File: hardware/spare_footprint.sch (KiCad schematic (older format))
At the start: 32 parts

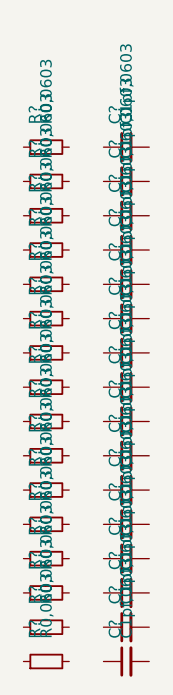
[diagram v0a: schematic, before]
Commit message: update,
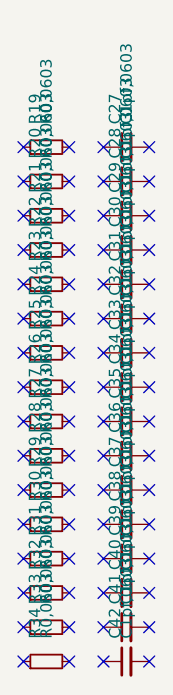
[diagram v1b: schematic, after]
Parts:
- gave numbers to parts that had none: 32
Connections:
- no-connect marks 0 -> 64

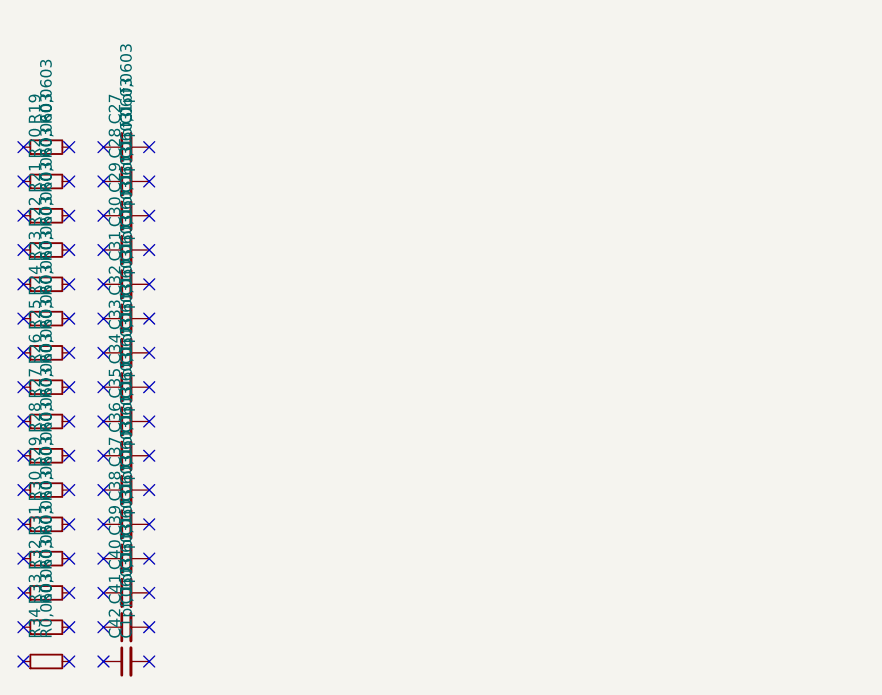
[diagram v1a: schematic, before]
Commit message: update,
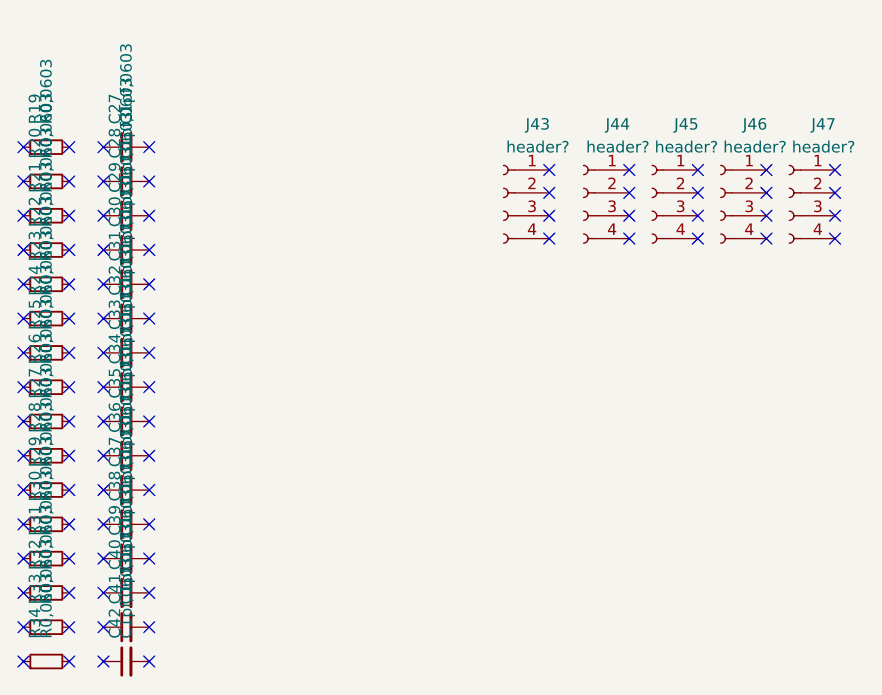
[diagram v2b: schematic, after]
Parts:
- added J43, J44, J45, J46, J47: header?, symbol Connector:Conn_01x04_Female
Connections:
- no-connect marks 64 -> 84
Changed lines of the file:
@@
 NoConn ~ 1650 3450
 NoConn ~ 1650 3600
+$Comp
+L Connector:Conn_01x04_Female J43
+U 1 1 5CFDD06D
+P 3550 1550
+F 0 "J43" H 3400 1850 50  0000 C CNN
+F 1 "header?" H 3400 1750 50  0000 C CNN
+F 2 "" H 3550 1550 50  0001 C CNN
+F 3 "~" H 3550 1550 50  0001 C CNN
+	1    3550 1550
+	-1   0    0    -1
+$EndComp
+NoConn ~ 3750 1450
+NoConn ~ 3750 1550
+NoConn ~ 3750 1650
+NoConn ~ 3750 1750
+$Comp
+L Connector:Conn_01x04_Female J44
+U 1 1 5CFDE011
+P 3900 1550
+F 0 "J44" H 3750 1850 50  0000 C CNN
+F 1 "header?" H 3750 1750 50  0000 C CNN
+F 2 "" H 3900 1550 50  0001 C CNN
+F 3 "~" H 3900 1550 50  0001 C CNN
+	1    3900 1550
+	-1   0    0    -1
+$EndComp
+NoConn ~ 4100 1450
+NoConn ~ 4100 1550
+NoConn ~ 4100 1650
+NoConn ~ 4100 1750
+$Comp
+L Connector:Conn_01x04_Female J45
+U 1 1 5CFDE347
+P 4200 1550
+F 0 "J45" H 4050 1850 50  0000 C CNN
+F 1 "header?" H 4050 1750 50  0000 C CNN
+F 2 "" H 4200 1550 50  0001 C CNN
+F 3 "~" H 4200 1550 50  0001 C CNN
+	1    4200 1550
+	-1   0    0    -1
+$EndComp
+NoConn ~ 4400 1450
+NoConn ~ 4400 1550
+NoConn ~ 4400 1650
+NoConn ~ 4400 1750
+$Comp
+L Connector:Conn_01x04_Female J46
+U 1 1 5CFDE710
+P 4500 1550
+F 0 "J46" H 4350 1850 50  0000 C CNN
+F 1 "header?" H 4350 1750 50  0000 C CNN
+F 2 "" H 4500 1550 50  0001 C CNN
+F 3 "~" H 4500 1550 50  0001 C CNN
+	1    4500 1550
+	-1   0    0    -1
+$EndComp
+NoConn ~ 4700 1450
+NoConn ~ 4700 1550
+NoConn ~ 4700 1650
+NoConn ~ 4700 1750
+$Comp
+L Connector:Conn_01x04_Female J47
+U 1 1 5CFDF291
+P 4800 1550
+F 0 "J47" H 4650 1850 50  0000 C CNN
+F 1 "header?" H 4650 1750 50  0000 C CNN
+F 2 "" H 4800 1550 50  0001 C CNN
+F 3 "~" H 4800 1550 50  0001 C CNN
+	1    4800 1550
+	-1   0    0    -1
+$EndComp
+NoConn ~ 5000 1450
+NoConn ~ 5000 1550
+NoConn ~ 5000 1650
+NoConn ~ 5000 1750
 $EndSCHEMATC
